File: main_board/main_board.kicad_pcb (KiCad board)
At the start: 2 copper layers, 146 x 111.8 mm, 128 parts, among them J1 stepper 0, J10 24VDC output 5, J11 5VDC output 0, J12 5VDC output 1, J13 5VDC output 2, J14 5VDC output 3, J15 5VDC output 4, J16 5VDC output 5, J17 temperature measure 0, J18 temperature measure 1, J19 I2C, J2 stepper 1, J20 I2C, J21 I2C, J22 I2C, J23 hall measure 0, J24 weight measure 0, J25 light measure 0, J26 24VDC_in, J27 24VDC to 5VDC step down, J28 24VDC, J29 24VDC, J3 stepper 2, J30 24VDC, J31 5VDC, J32 5VDC, J33 5VDC, J34 hall measure 1, J35 reflective sensor 0, J36 24VDC, J37 24VDC, J38 24VDC, J39 5VDC, J4 stepper 3, J40 5VDC, J41 5VDC, J42 Conn_01x05_Male, J5 24VDC output 0, J6 24VDC output 1, J7 24VDC output 2, J8 24VDC output 3, J9 24VDC output 4, Q1 Q_NMOS_GDS, Q10 BS170, Q11 BS170, Q12 BS170, Q2 Q_NMOS_GDS, Q3 Q_NMOS_GDS, Q4 Q_NMOS_GDS, Q5 Q_NMOS_GDS, Q6 Q_NMOS_GDS, Q7 BS170, Q8 BS170, Q9 BS170, U1 ESP32-DEVKITC-32D, U2 PCA9685PW

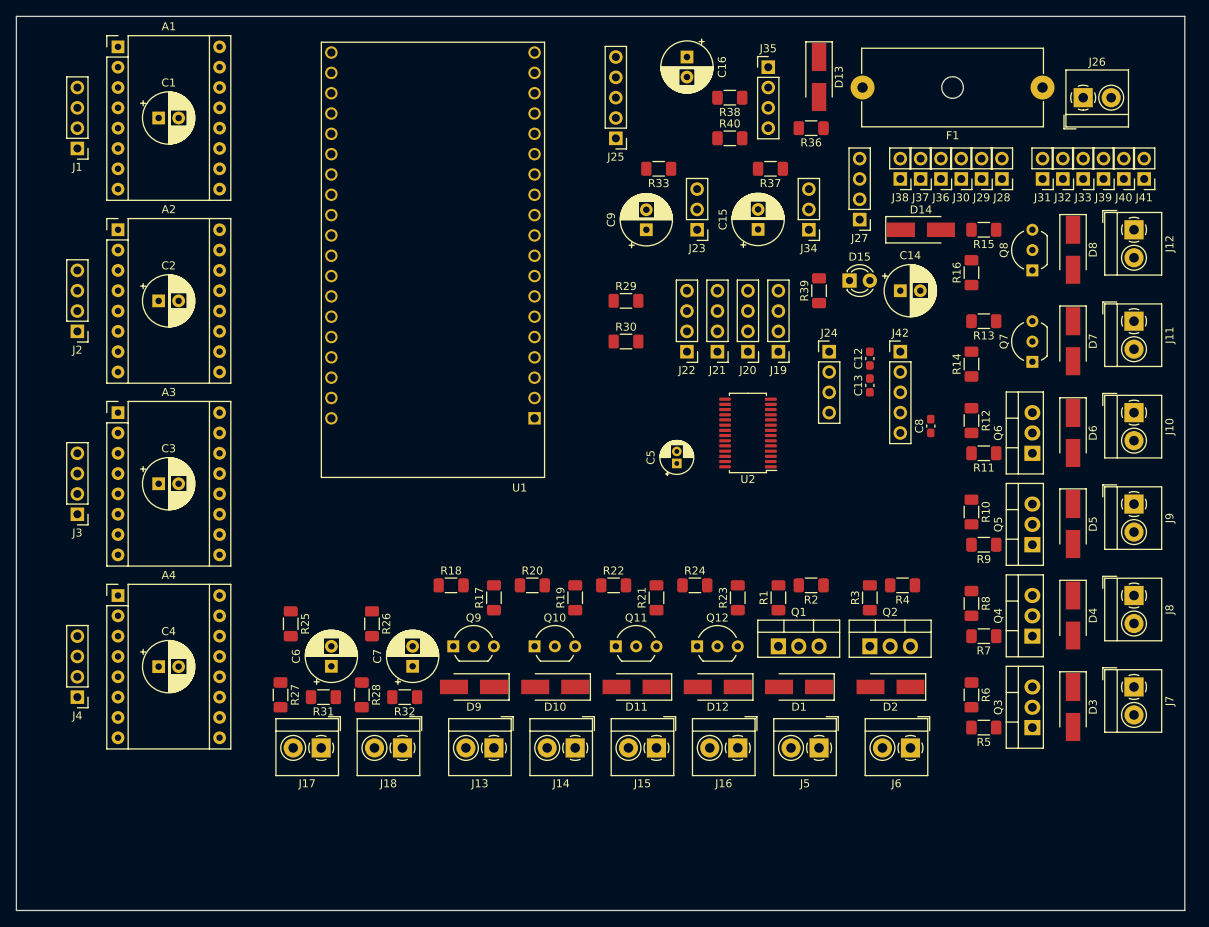
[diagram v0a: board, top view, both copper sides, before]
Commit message: routs added
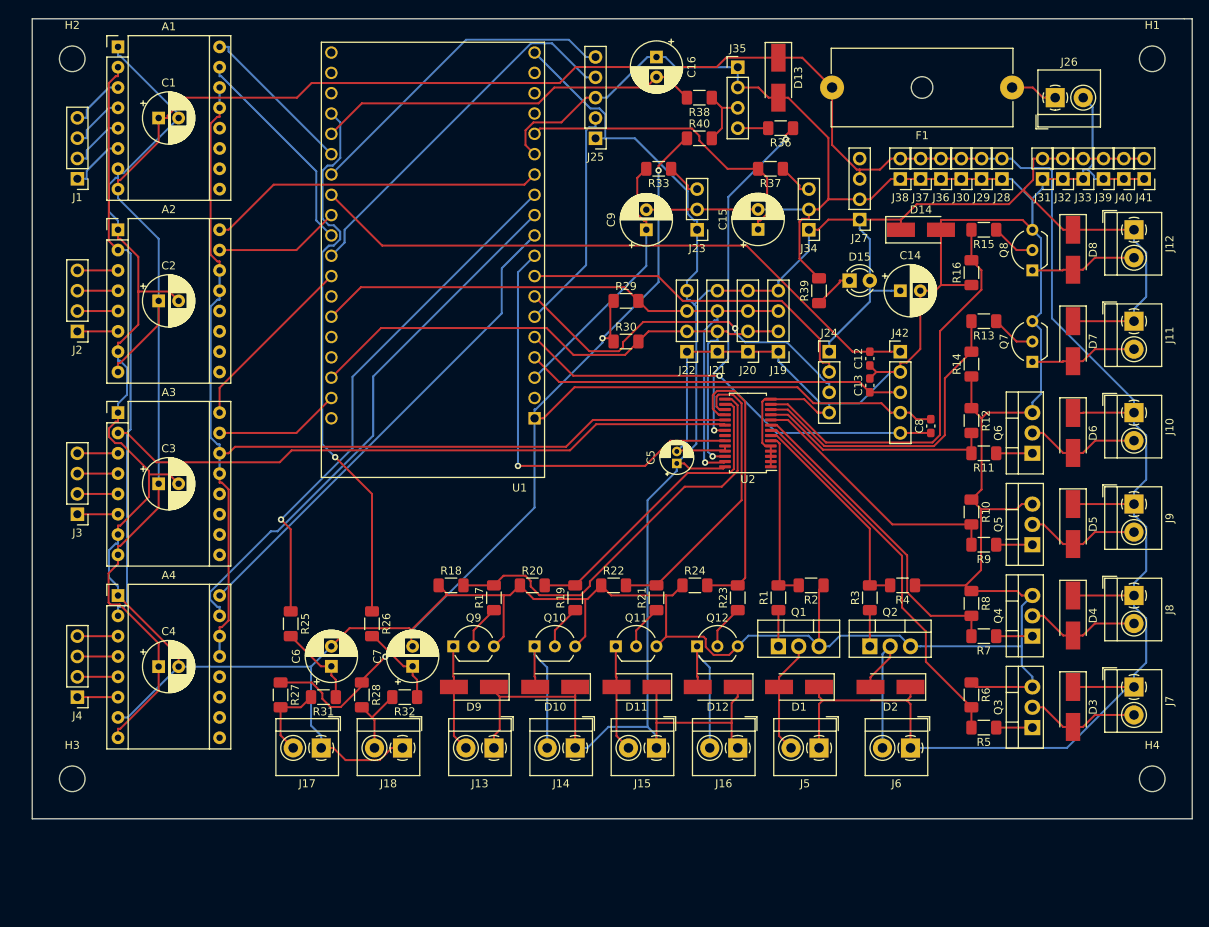
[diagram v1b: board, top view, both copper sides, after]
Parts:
- added H1: MountingHole, MountingHole:MountingHole_3.2mm_M3, F.Cu at (175.0, 18.0)
- added H2: MountingHole, MountingHole:MountingHole_3.2mm_M3, F.Cu at (40.0, 18.0)
- added H3: MountingHole, MountingHole:MountingHole_3.2mm_M3, F.Cu at (40.0, 108.0)
- added H4: MountingHole, MountingHole:MountingHole_3.2mm_M3, F.Cu at (175.0, 108.0)
- moved D13 5.08 mm to (128.3, 20.4)
- moved C16 3.81 mm to (113.0, 17.8)
- moved F1 3.81 mm to (157.5, 21.6)
- moved J35 3.81 mm to (123.2, 19.1)
- moved R36 3.81 mm to (128.6, 26.7)
- moved R38 3.81 mm to (118.4, 22.9)
- moved R40 3.81 mm to (118.4, 27.9)
- moved J1 3.79 mm to (40.6, 33.0)
- moved J26 3.50 mm to (162.9, 22.9)
- moved J25 2.54 mm to (105.4, 27.9)
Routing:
- net GND: track 0.00 -> 658.6 mm
- net +24V: track 0.00 -> 389.9 mm
- net +5V: track 0.00 -> 299.4 mm
- net +3V3: track 0.00 -> 157.6 mm, vias 0 -> 3
- net stepperErr: track 0.00 -> 152.6 mm
- net stepperON: track 0.00 -> 139.8 mm
- net SDA: track 0.00 -> 81.1 mm, vias 0 -> 1
- net SCL: track 0.00 -> 79.7 mm, vias 0 -> 1
- net enca: track 0.00 -> 79.2 mm
- net Net-(R26-Pad1): track 0.00 -> 69.1 mm, vias 0 -> 1
- net STEP3: track 0.00 -> 68.0 mm
- net Net-(R25-Pad1): track 0.00 -> 65.7 mm, vias 0 -> 1
- net DIR3: track 0.00 -> 61.3 mm
- net button: track 0.00 -> 54.5 mm, vias 0 -> 1
- net OE: track 0.00 -> 54.3 mm, vias 0 -> 1
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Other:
- board size 146 x 111.8 mm -> 145 x 100 mm
